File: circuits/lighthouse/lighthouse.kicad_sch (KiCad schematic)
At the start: 53 parts, among them J1 USB_C_Receptacle_USB2.0_14P, J2 Conn_01x03_Socket, Q1 S9013, Q4 SS8050, Q5 SS8050, U10 CP2102-GMR, U2 AMS1117-3.3, U7 ESP32-WROOM-32

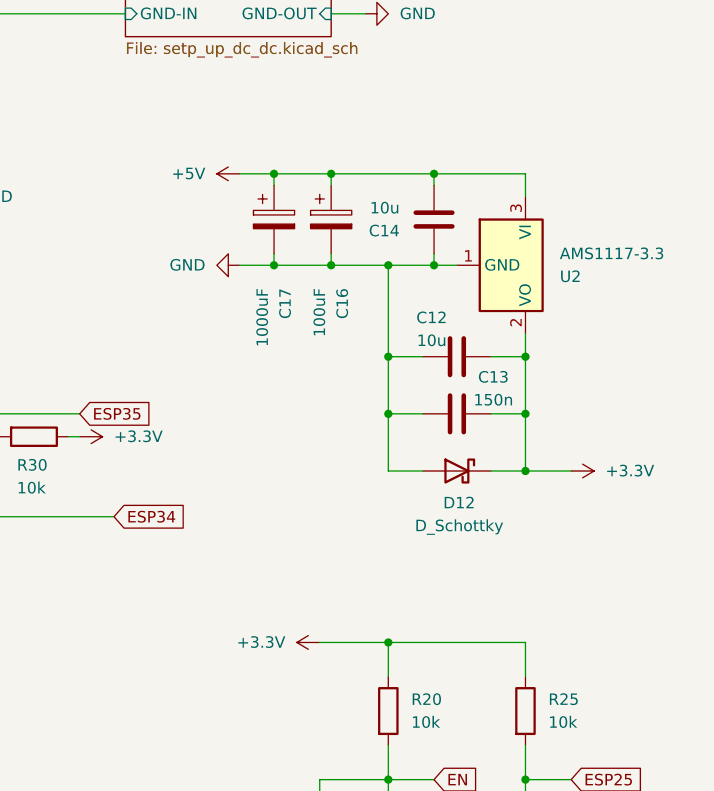
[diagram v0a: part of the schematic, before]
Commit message: Production ready? (most likely not)
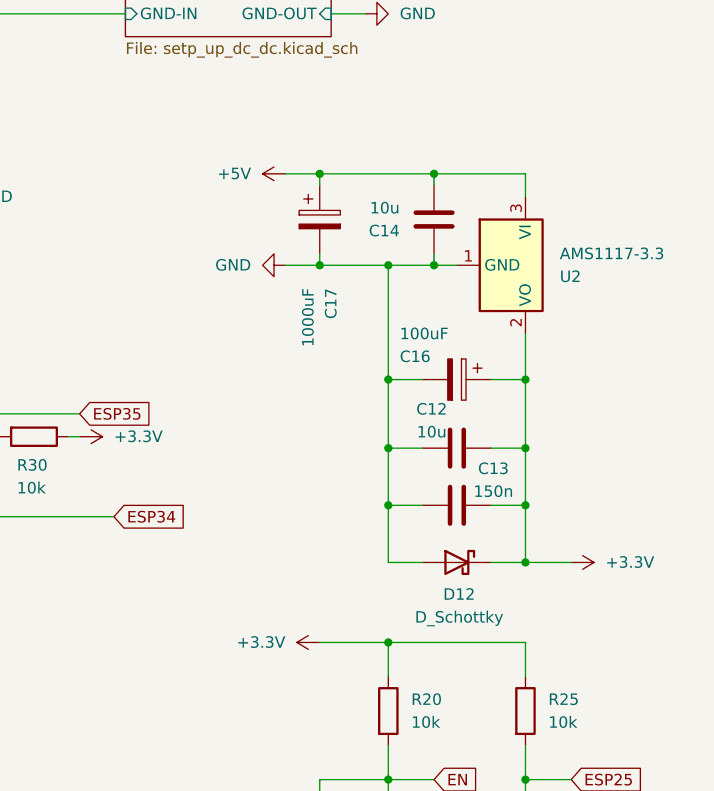
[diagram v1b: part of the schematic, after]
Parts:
- D15, D16: footprint Diode_SMD:D_2114_3652Metric_Pad1.85x3.75mm_HandSolder -> Diode_SMD:D_SMA
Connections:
- net +3.3V: now also C16.1
- net +5V: no longer C16.1
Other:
- moved on the sheet: C12, C13, C16, C17, D12
